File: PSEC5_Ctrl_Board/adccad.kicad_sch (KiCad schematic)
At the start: 10 parts, among them U2 LTC2600CGN_PBF, U4 LTC2600CGN_PBF

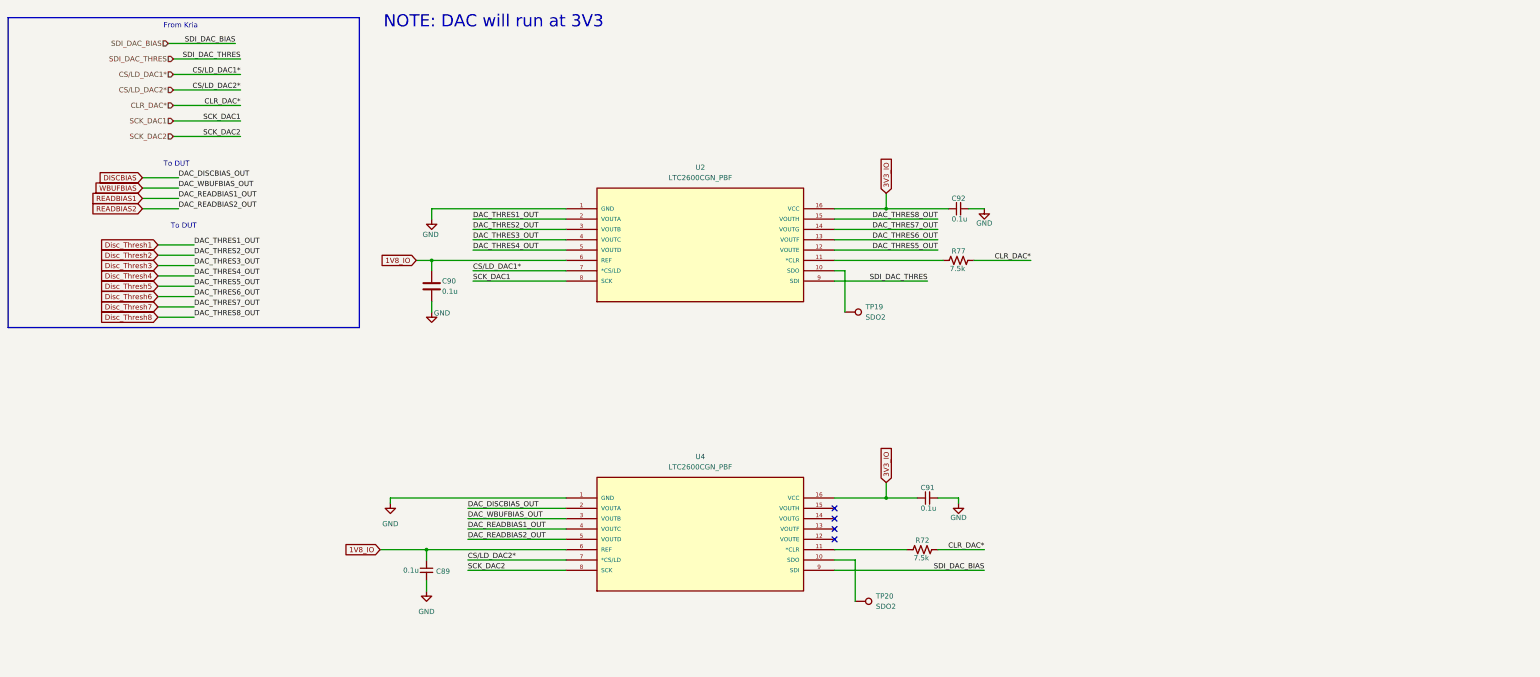
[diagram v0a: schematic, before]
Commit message: ERC "Done" (4 errors left) Schematic "Done"
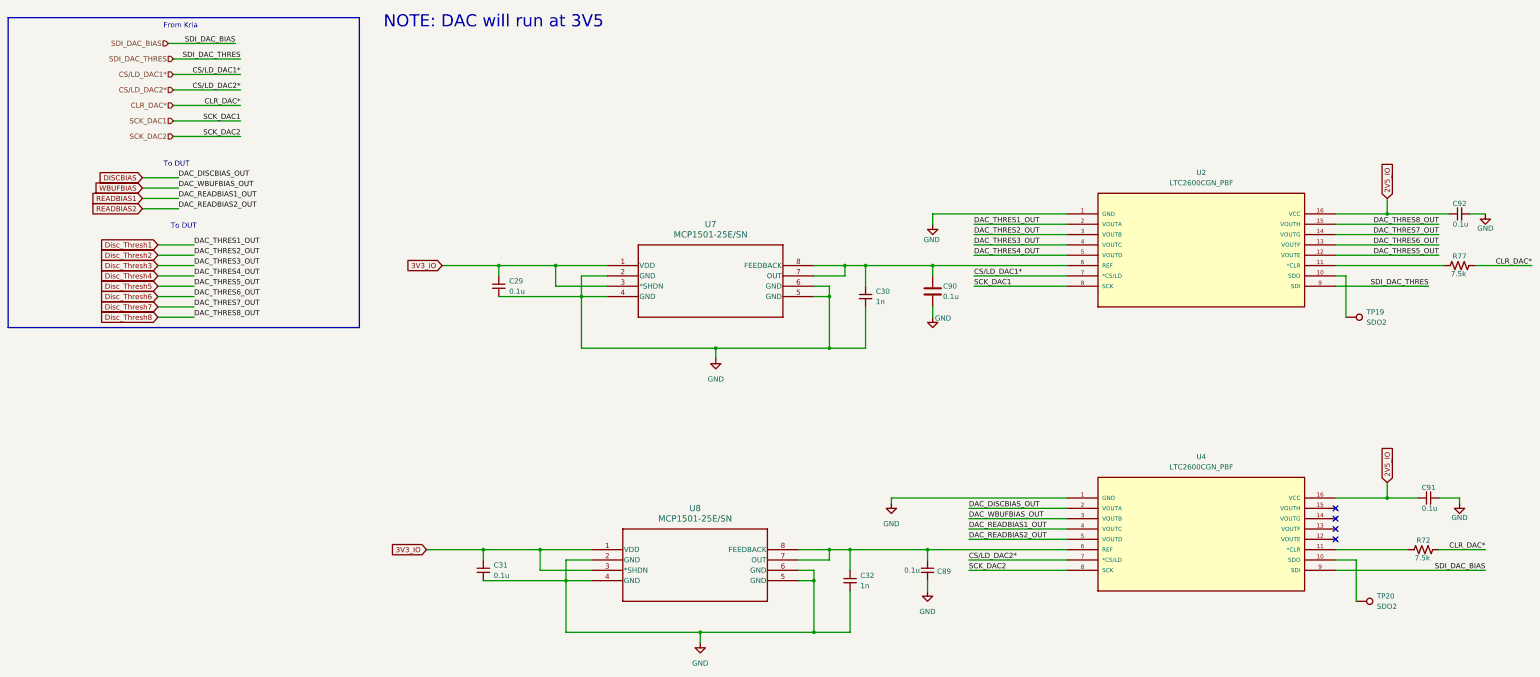
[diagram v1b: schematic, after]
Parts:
- added C29, C31: 0.1u, Capacitor_SMD:C_0603_1608Metric, symbol Device:C_Small
- added C30, C32: 1n, Capacitor_SMD:C_0603_1608Metric, symbol Device:C_Small
- added U7, U8: MCP1501-25E/SN, SOIC8_NARROW_SN_MCH, symbol PSEC5_ctrlbd:MCP1501-25E_SN
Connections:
- net 3V3_IO: now also C29.1, C31.1, U7.1 (VDD), U7.3 (*SHDN), U8.1 (VDD), U8.3 (*SHDN); no longer C91.1, C92.1, U2.16 (VCC), U4.16 (VCC)
- net GND: now also C29.2, C30.2, C31.2, C32.2, U7.2 (GND), U7.4 (GND), U7.5 (GND), U7.6 (GND), U8.2 (GND), U8.4 (GND), U8.5 (GND), U8.6 (GND)
- net 1V8_IO: no longer names the net of C90.1, U2.6 (REF)
- net 1V8_IO: now also C30.1, U7.7 (OUT), U7.8 (FEEDBACK); no longer C89.1, U4.6 (REF)
- new net: C32.1, C89.1, U4.6 (REF), U8.7 (OUT), U8.8 (FEEDBACK)
- new net 2V5_IO: C91.1, C92.1, U2.16 (VCC), U4.16 (VCC)
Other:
- note added: "NOTE: DAC will run at 3V5"
- note removed: "NOTE: DAC will run at 3V3"
- moved on the sheet: C89, C90, C91, C92, R72, R77, TP19, TP20, U2, U4
